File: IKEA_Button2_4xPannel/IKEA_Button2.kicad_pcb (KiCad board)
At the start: 2 copper layers, 99.5 x 100 mm, 166 parts, among them Q1 2N7002ET, U1 ICC-1

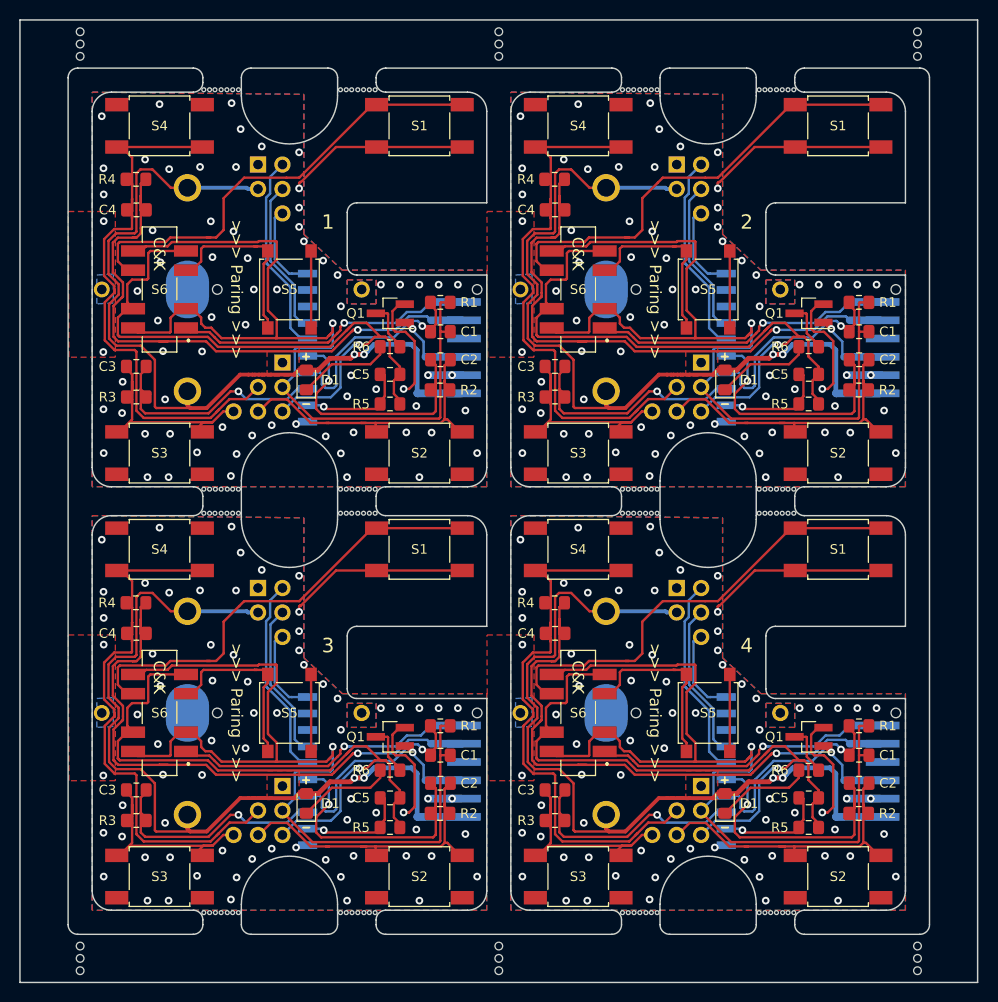
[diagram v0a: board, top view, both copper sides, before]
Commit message: update
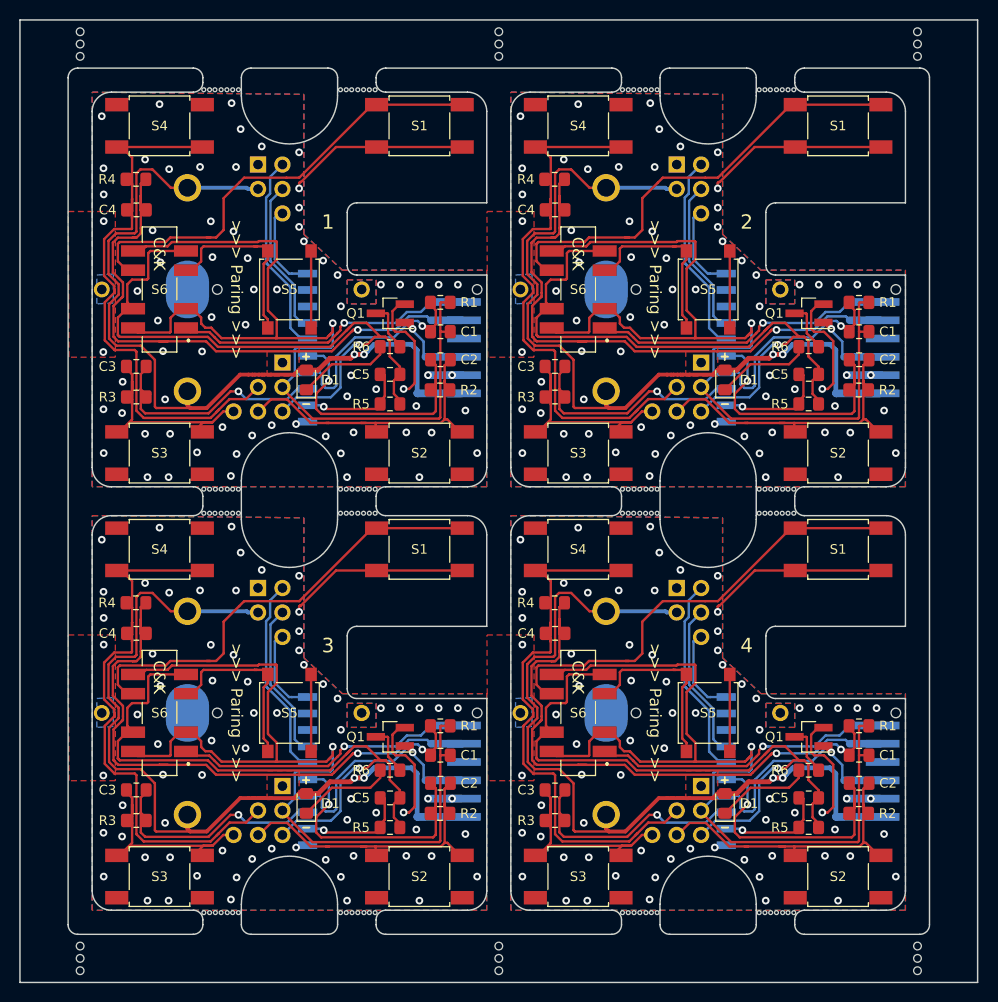
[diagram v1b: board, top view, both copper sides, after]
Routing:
- net Net-(SWDIO1-Pad1): vias 2 -> 0
- net GND: vias 284 -> 288
- net (no net): vias 2 -> 0
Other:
- net class Default removed
